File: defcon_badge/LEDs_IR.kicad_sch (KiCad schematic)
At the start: 13 parts, among them U30 TSOP4838

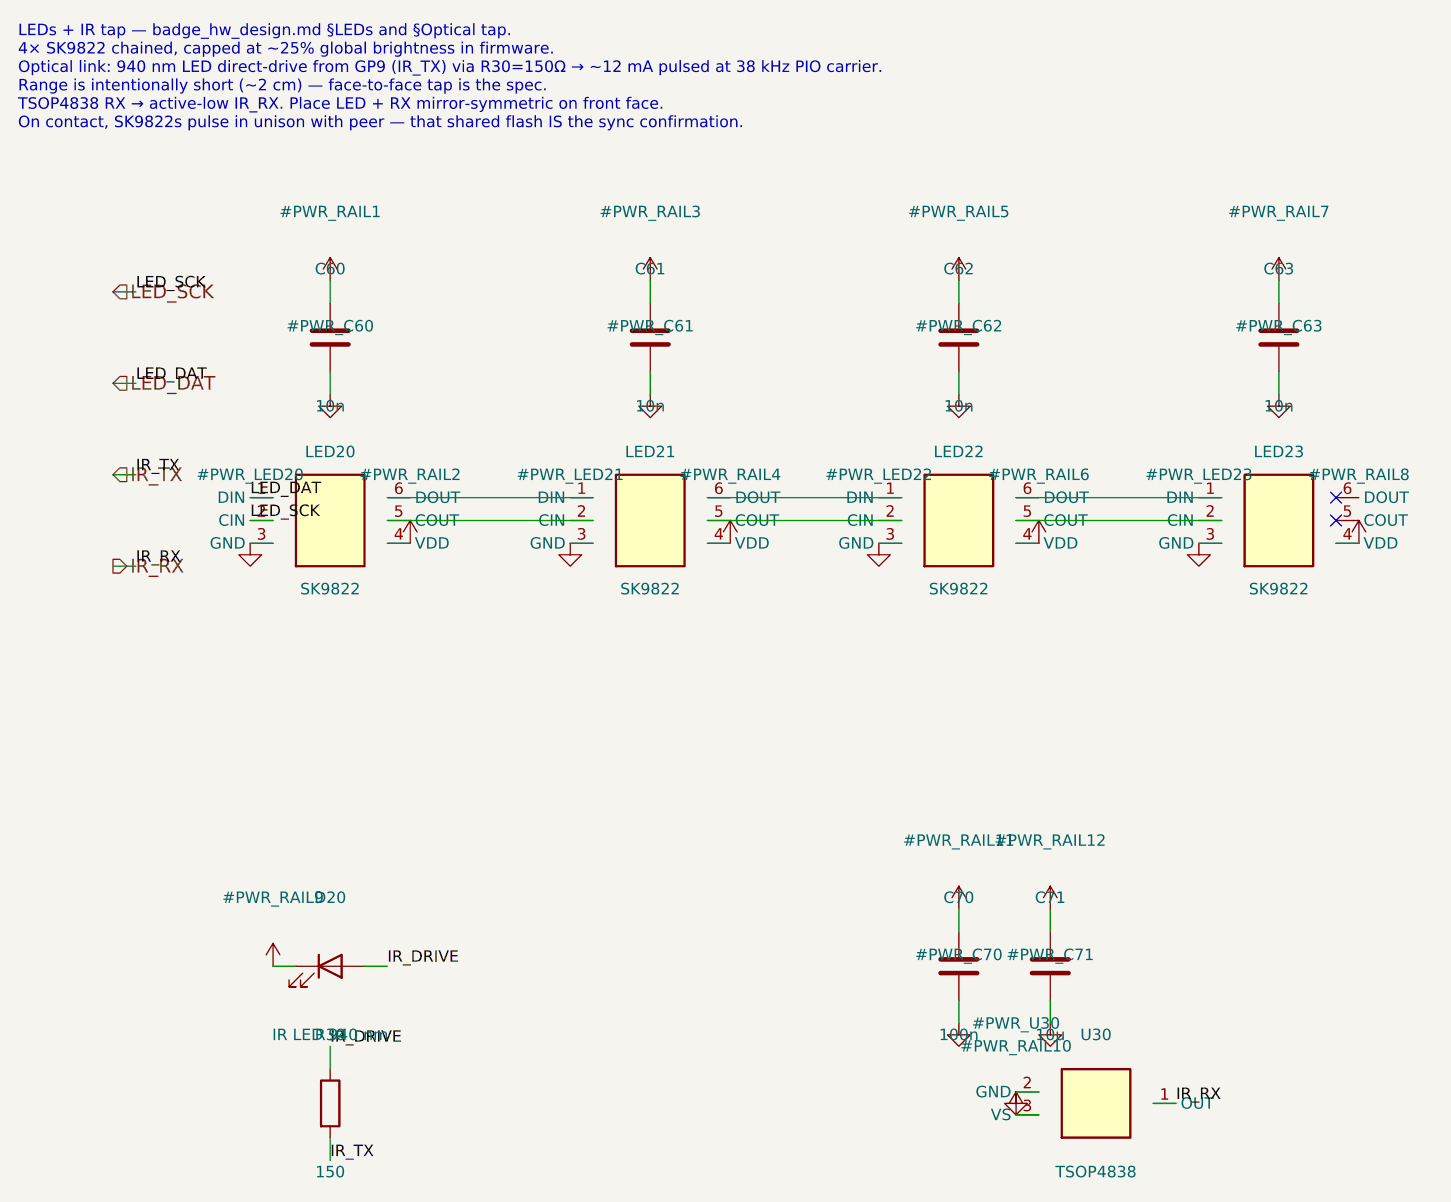
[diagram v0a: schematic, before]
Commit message: Routing redo
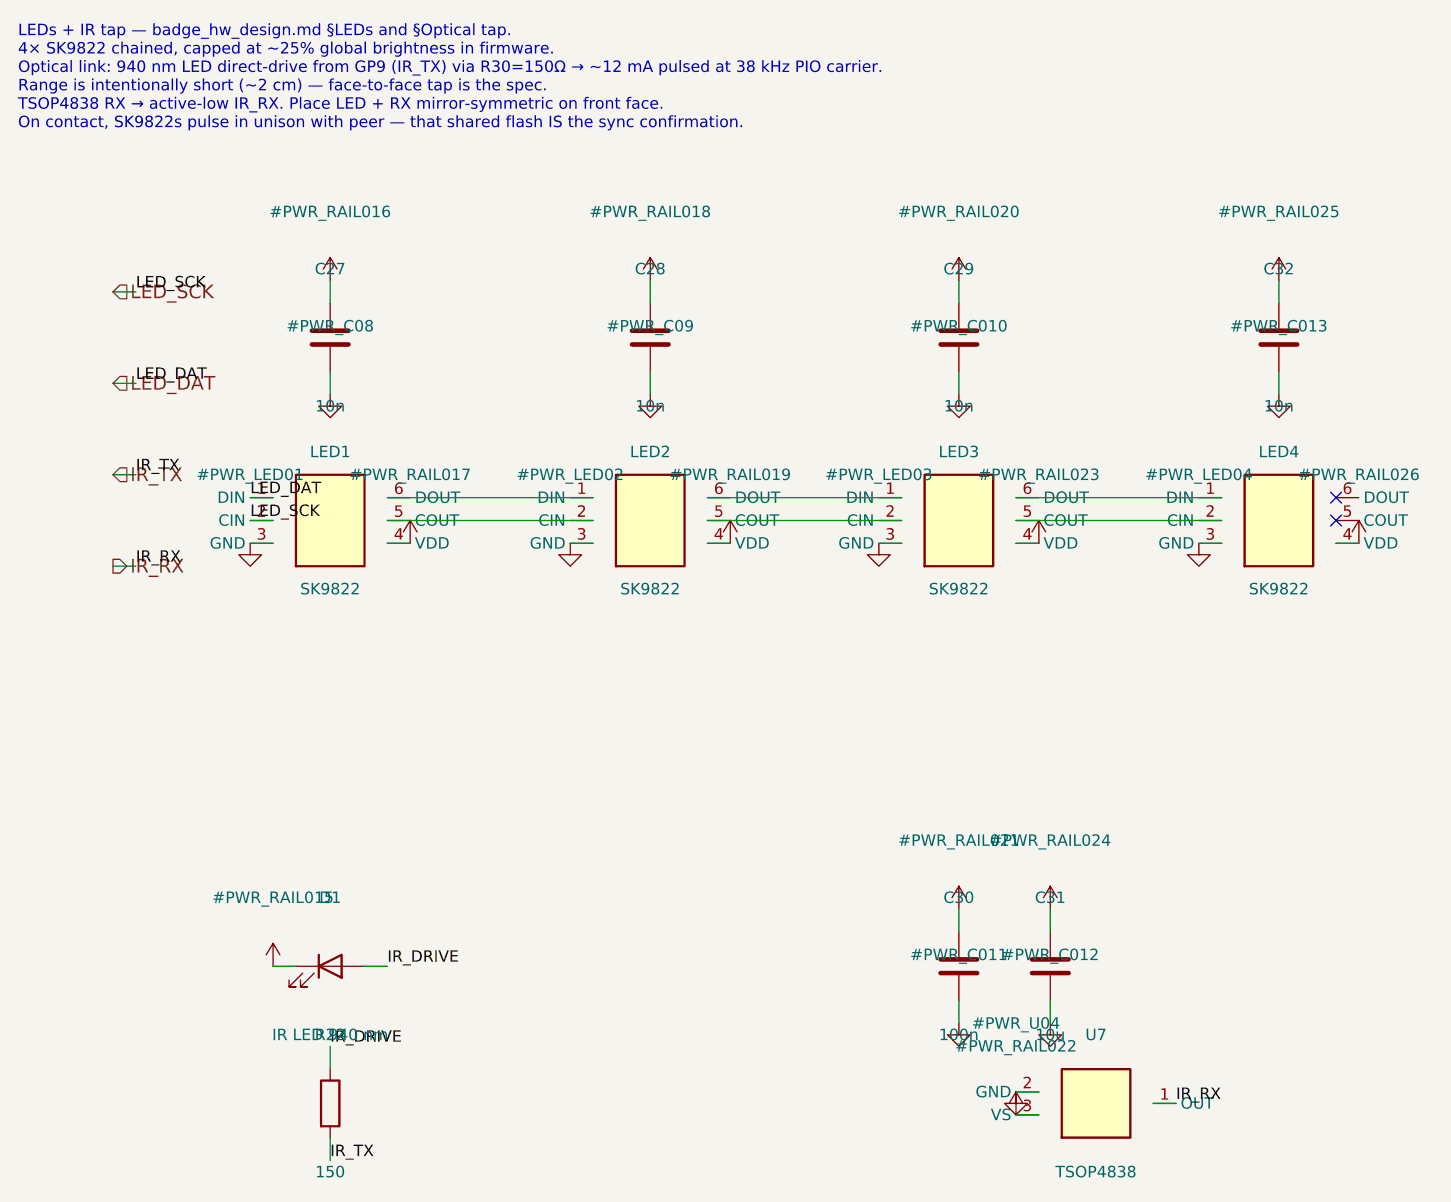
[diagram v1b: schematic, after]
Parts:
- renumbered C60 to C27, C61 to C28, C62 to C29, C70 to C30, C71 to C31, C63 to C32, D20 to D1, LED20 to LED1, LED21 to LED2, LED22 to LED3, LED23 to LED4, R30 to R22, U30 to U7
